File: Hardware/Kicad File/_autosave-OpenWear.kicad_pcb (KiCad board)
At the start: 4 copper layers, 50 x 50 mm, 41 parts, among them J1 USB_C, J2 Connector, Q1 BC847B, Q2 DMG3415U, U1 ESP32-PICO-D4, U2 BMP280, U3 CH343P, U4 TLV70233_SOT23-5, U5 MCP73831-2-OT, U6 LSM6DS3

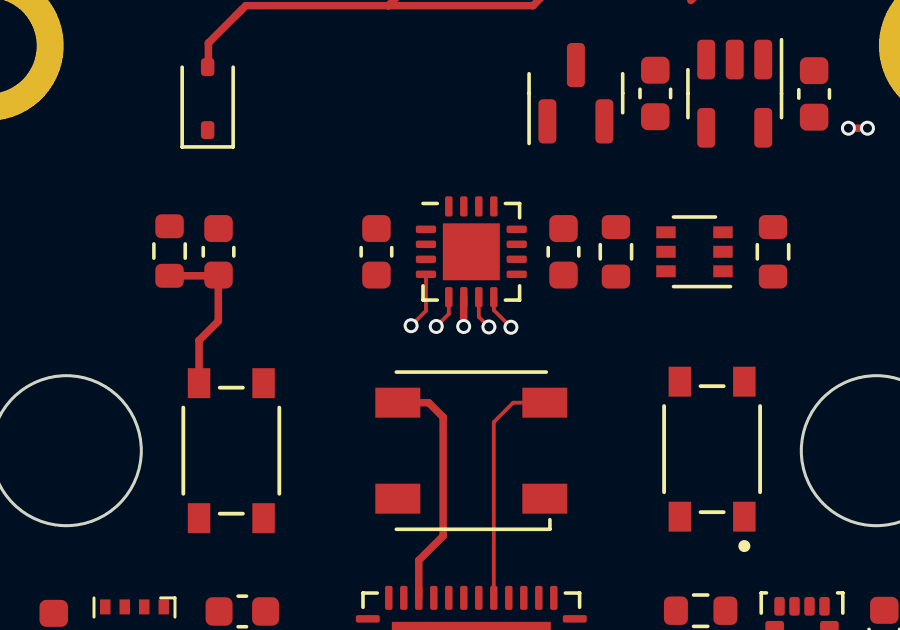
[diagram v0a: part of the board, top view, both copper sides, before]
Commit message: update sch
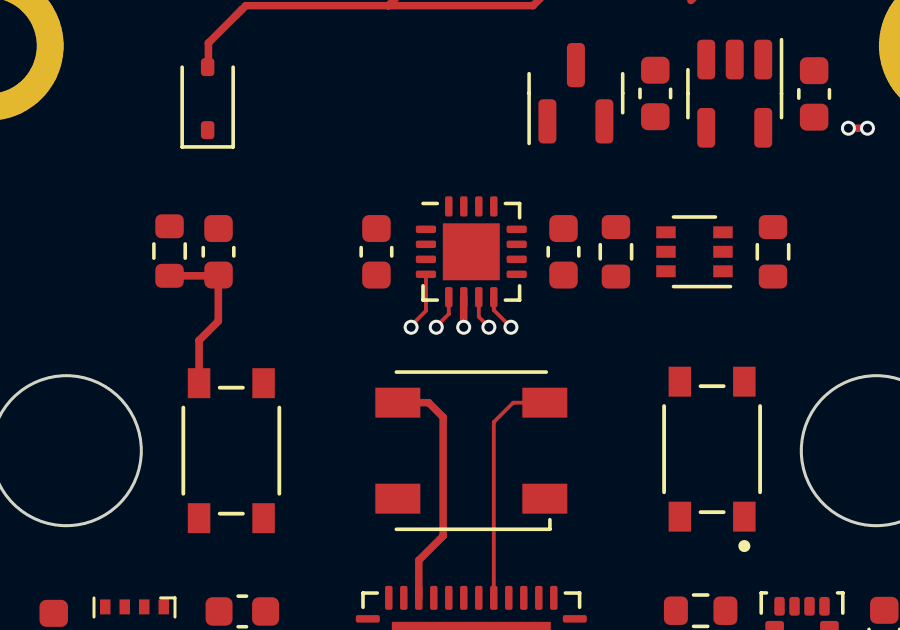
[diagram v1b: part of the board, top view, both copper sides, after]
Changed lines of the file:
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@@
   (segment (start 142.3546 75.2934) (end 142.126 75.522) (width 0.25) (layer "F.Cu") (net 2))
   (segment (start 147.2314 75.1664) (end 142.4816 75.1664) (width 0.25) (layer "F.Cu") (net 2))
-  (segment (start 150.25 84.8831) (end 150.25 85.539893) (width 0.127) (layer "F.Cu") (net 4))
+  (segment (start 150.25 85.539893) (end 150.25 84.8831) (width 0.127) (layer "F.Cu") (net 4))
   (segment (start 150.25 70.954) (end 150.254 70.95) (width 0.2) (layer "F.Cu") (net 4))
   (segment (start 150.25 73.2018) (end 150.25 70.954) (width 0.127) (layer "F.Cu") (net 4))
-  (segment (start 150.25 85.539893) (end 150.585966 85.875859) (width 0.127) (layer "F.Cu") (net 4))
+  (segment (start 150.585966 85.875859) (end 150.25 85.539893) (width 0.127) (layer "F.Cu") (net 4))
   (segment (start 149.25 71.446) (end 149.746 70.95) (width 0.127) (layer "F.Cu") (net 4))
   (segment (start 149.746 70.95) (end 150.254 70.95) (width 0.127) (layer "F.Cu") (net 4))
   (segment (start 149.25 73.2018) (end 149.25 71.446) (width 0.127) (layer "F.Cu") (net 4))
-  (via (at 150.585966 85.875859) (size 0.5) (drill 0.3) (layers "F.Cu" "B.Cu") (net 4))
+  (via (at 150.585966 85.8852) (size 0.5) (drill 0.3) (layers "F.Cu" "B.Cu") (net 4))
   (via (at 150.254 70.95) (size 0.5) (drill 0.3) (layers "F.Cu" "B.Cu") (net 4))
+  (segment (start 149.2325 72.127899) (end 149.2325 71.4635) (width 0.127) (layer "In2.Cu") (net 4))
+  (segment (start 150.5842 85.874093) (end 150.5842 73.479599) (width 0.127) (layer "In2.Cu") (net 4))
   (segment (start 150.5842 73.479599) (end 149.2325 72.127899) (width 0.127) (layer "In2.Cu") (net 4))
   (segment (start 149.2325 71.4635) (end 149.746 70.95) (width 0.127) (layer "In2.Cu") (net 4))
-  (segment (start 150.5842 85.874093) (end 150.5842 73.479599) (width 0.127) (layer "In2.Cu") (net 4))
+  (segment (start 150.585966 85.875859) (end 150.5842 85.874093) (width 0.127) (layer "In2.Cu") (net 4))
   (segment (start 149.746 70.95) (end 150.254 70.95) (width 0.127) (layer "In2.Cu") (net 4))
-  (segment (start 150.585966 85.875859) (end 150.5842 85.874093) (width 0.127) (layer "In2.Cu") (net 4))
-  (segment (start 149.2325 72.127899) (end 149.2325 71.4635) (width 0.127) (layer "In2.Cu") (net 4))
   (segment (start 149.75 73.2018) (end 149.75 71.97) (width 0.127) (layer "F.Cu") (net 5))
   (segment (start 151.3208 85.8852) (end 150.75 85.3144) (width 0.127) (layer "F.Cu") (net 5))
@@
   (segment (start 162.557176 79.237775) (end 162.570516 79.251115) (width 0.254) (layer "F.Cu") (net 8))
   (via (at 162.570516 79.251115) (size 0.5) (drill 0.3) (layers "F.Cu" "B.Cu") (net 8))
-  (via (at 149.746 85.8598) (size 0.5) (drill 0.3) (layers "F.Cu" "B.Cu") (free) (net 8))
+  (via (at 149.746 85.8852) (size 0.5) (drill 0.3) (layers "F.Cu" "B.Cu") (free) (net 8))
   (via (at 163.205516 79.251115) (size 0.5) (drill 0.3) (layers "F.Cu" "B.Cu") (net 8))
   (segment (start 147.75 110.672) (end 147.4416 110.9804) (width 0.25) (layer "F.Cu") (net 9))
@@
   (segment (start 148.4875 84.1206) (end 148.4875 85.3403) (width 0.127) (layer "F.Cu") (net 63))
   (segment (start 148.4875 85.3403) (end 147.9934 85.8344) (width 0.127) (layer "F.Cu") (net 63))
-  (via (at 147.9934 85.8344) (size 0.5) (drill 0.3) (layers "F.Cu" "B.Cu") (net 63))
+  (via (at 147.9934 85.8852) (size 0.5) (drill 0.3) (layers "F.Cu" "B.Cu") (net 63))
   (segment (start 149.25 84.8831) (end 149.25 85.4414) (width 0.127) (layer "F.Cu") (net 64))
   (segment (start 149.25 85.4414) (end 148.8316 85.8598) (width 0.127) (layer "F.Cu") (net 64))
-  (via (at 148.8316 85.8598) (size 0.5) (drill 0.3) (layers "F.Cu" "B.Cu") (net 64))
+  (via (at 148.8316 85.8852) (size 0.5) (drill 0.3) (layers "F.Cu" "B.Cu") (net 64))
   (zone (net 1) (net_name "GND") (layers "F.Cu" "In1.Cu" "In2.Cu" "B.Cu") (hatch edge 0.5)
     (connect_pads (clearance 0))
